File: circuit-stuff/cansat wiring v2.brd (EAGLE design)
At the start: 100 x 26.7 mm, 6 parts

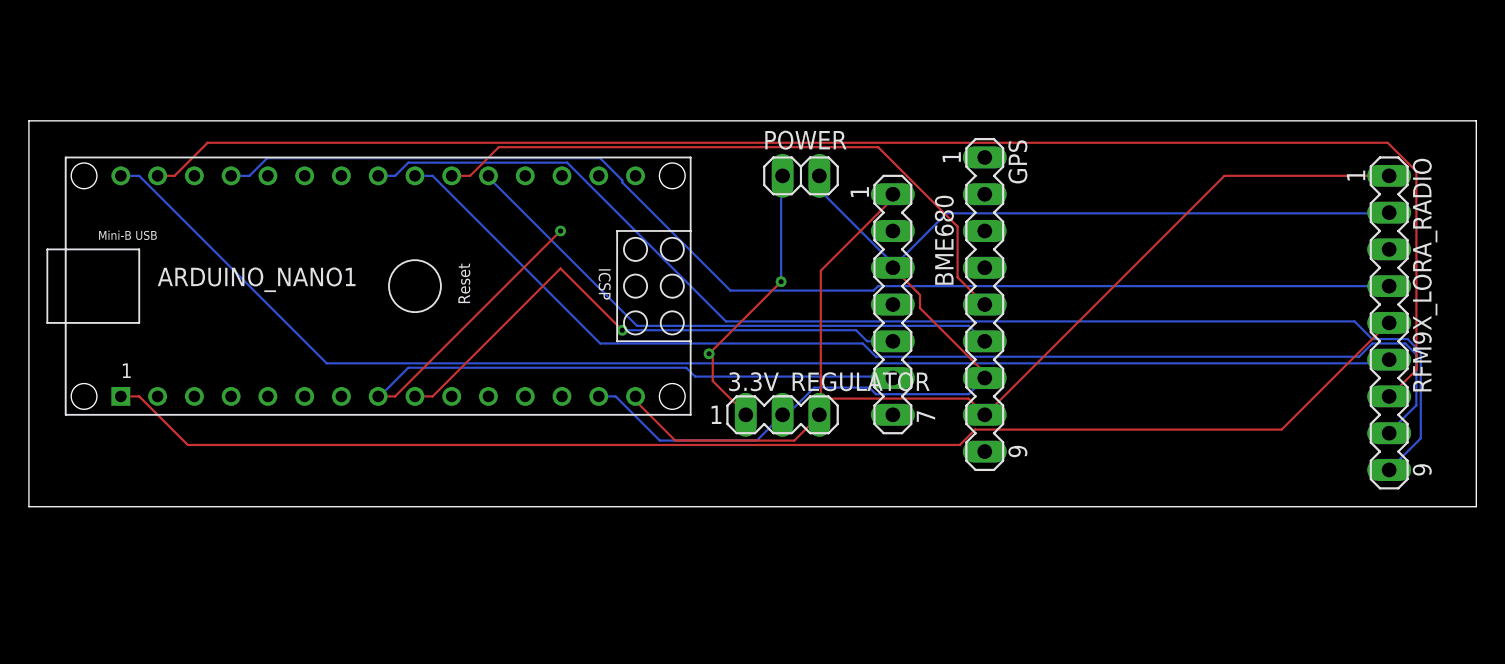
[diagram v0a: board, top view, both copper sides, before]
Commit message: Add files via upload
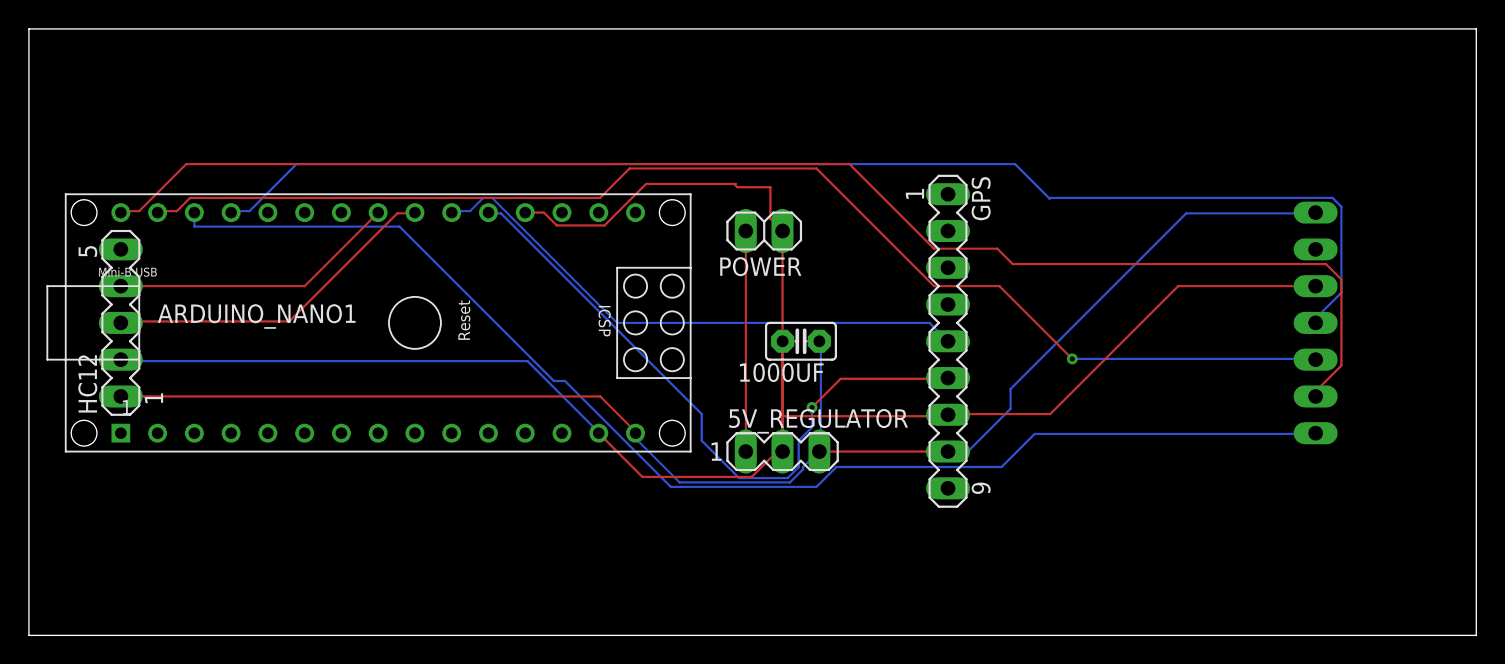
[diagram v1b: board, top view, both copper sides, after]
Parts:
- removed 3.3V_REGULATOR: (no value), con-lstb:MA03-1
- removed RFM9X_LORA_RADIO: (no value), con-lstb:MA09-1
- added 1000UF: (no value), capacitor-wima:C2.5-2
- added 5V_REGULATOR: (no value), con-lstb:MA03-1
- added HC12: (no value), con-lstb:MA05-1
- moved BME680 29.2 mm to (88.9, 66.0), flipped to the bottom
- moved POWER 4.58 mm to (50.8, 72.4), turned to 180 degrees
- moved GPS 3.59 mm to (63.5, 64.8)
- moved ARDUINO_NANO1 2.54 mm to (26.7, 66.0)
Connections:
- removed net GND: ARDUINO_NANO1.19
- removed net N$11: ARDUINO_NANO1.8, BME680.6
- removed net N$12: ARDUINO_NANO1.9, BME680.5
- net +: now also 1000UF.2, 5V_REGULATOR.2, ARDUINO_NANO1.19, HC12.2, POWER.1; no longer 3.3V_REGULATOR.2, POWER.2, RFM9X_LORA_RADIO.2
- net -: now also 5V_REGULATOR.1, POWER.2; no longer 3.3V_REGULATOR.1, POWER.1
- net N$1: now also ARDUINO_NANO1.27, BME680.4; no longer ARDUINO_NANO1.23, RFM9X_LORA_RADIO.9
- net N$2: now also ARDUINO_NANO1.29, BME680.5; no longer ARDUINO_NANO1.22, RFM9X_LORA_RADIO.8
- net N$4: now also 1000UF.1, 5V_REGULATOR.3, HC12.1; no longer 3.3V_REGULATOR.3, RFM9X_LORA_RADIO.1
- net N$6: now also ARDUINO_NANO1.30, BME680.6; no longer ARDUINO_NANO1.29, RFM9X_LORA_RADIO.7
- net N$7: now also ARDUINO_NANO1.23, HC12.4; no longer ARDUINO_NANO1.30, RFM9X_LORA_RADIO.6
- net N$8: now also ARDUINO_NANO1.28, BME680.7; no longer ARDUINO_NANO1.1, RFM9X_LORA_RADIO.5
- net N$9: now also ARDUINO_NANO1.22, HC12.3; no longer ARDUINO_NANO1.27, RFM9X_LORA_RADIO.4
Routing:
- net N$7: track 93.1 -> 19.9 mm
- net N$9: track 84.5 -> 23.5 mm
- net +: track 84.9 -> 142.9 mm
- net N$11: track 54.0 -> 0.00 mm, vias 1 -> 0
- net N$12: track 38.8 -> 0.00 mm, vias 1 -> 0
- net N$4: track 80.1 -> 101.7 mm
- net N$6: track 105.1 -> 97.9 mm
- net N$3: track 39.1 -> 45.2 mm, vias 0 -> 1
- net N$2: track 81.3 -> 86.7 mm, vias 0 -> 1
- net N$5: track 44.2 -> 38.8 mm
- net N$8: track 92.6 -> 87.4 mm
- net -: track 20.1 -> 15.2 mm, vias 2 -> 0
- net N$1: track 86.9 -> 88.1 mm
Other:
- board size 100 x 26.7 mm -> 100 x 41.9 mm
